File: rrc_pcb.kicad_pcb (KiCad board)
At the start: 2 copper layers, 139 x 50.8 mm, 13 parts, among them J1 Voltage Regulator Input, J2 Conn_01x03_Male, U1 ADXL357Z, U2 Teensy3.6-teensy, U3 BN220-GPS, U4 MS5611, U5 logo

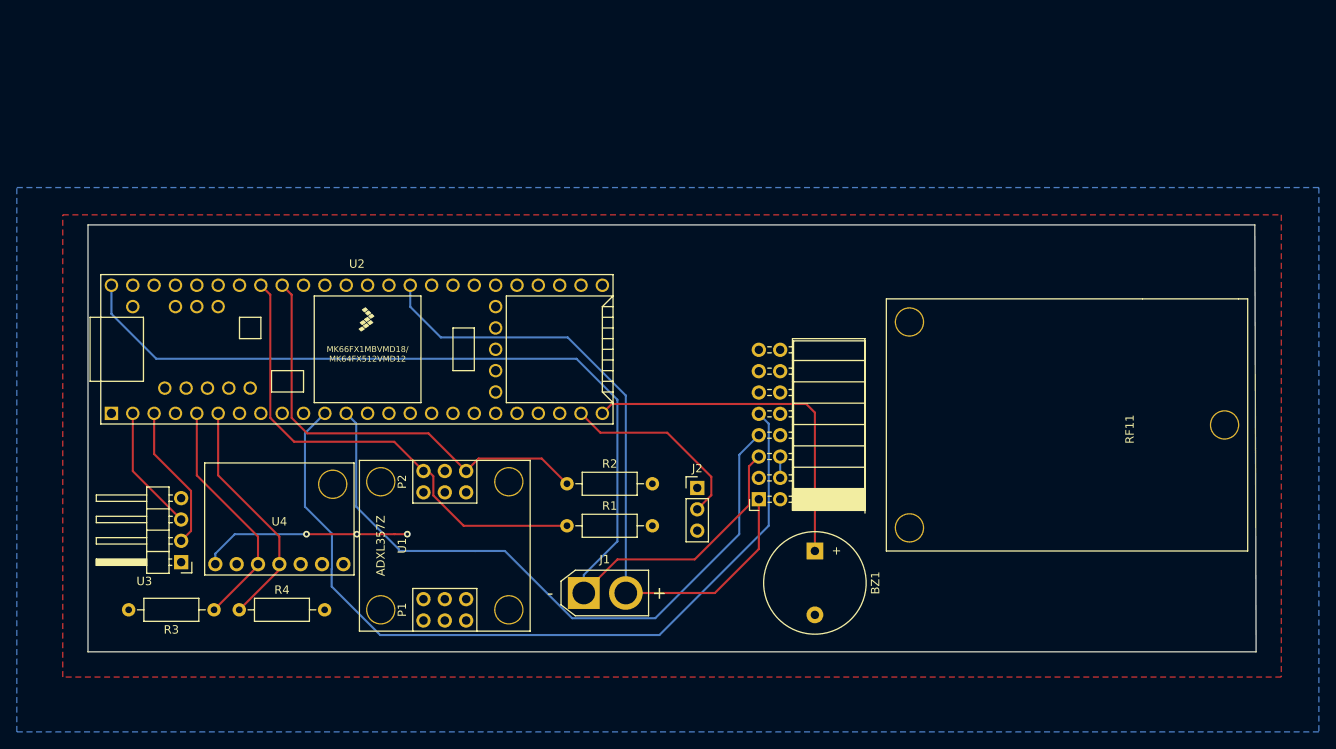
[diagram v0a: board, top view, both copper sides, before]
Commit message: fixed pcb trace issues
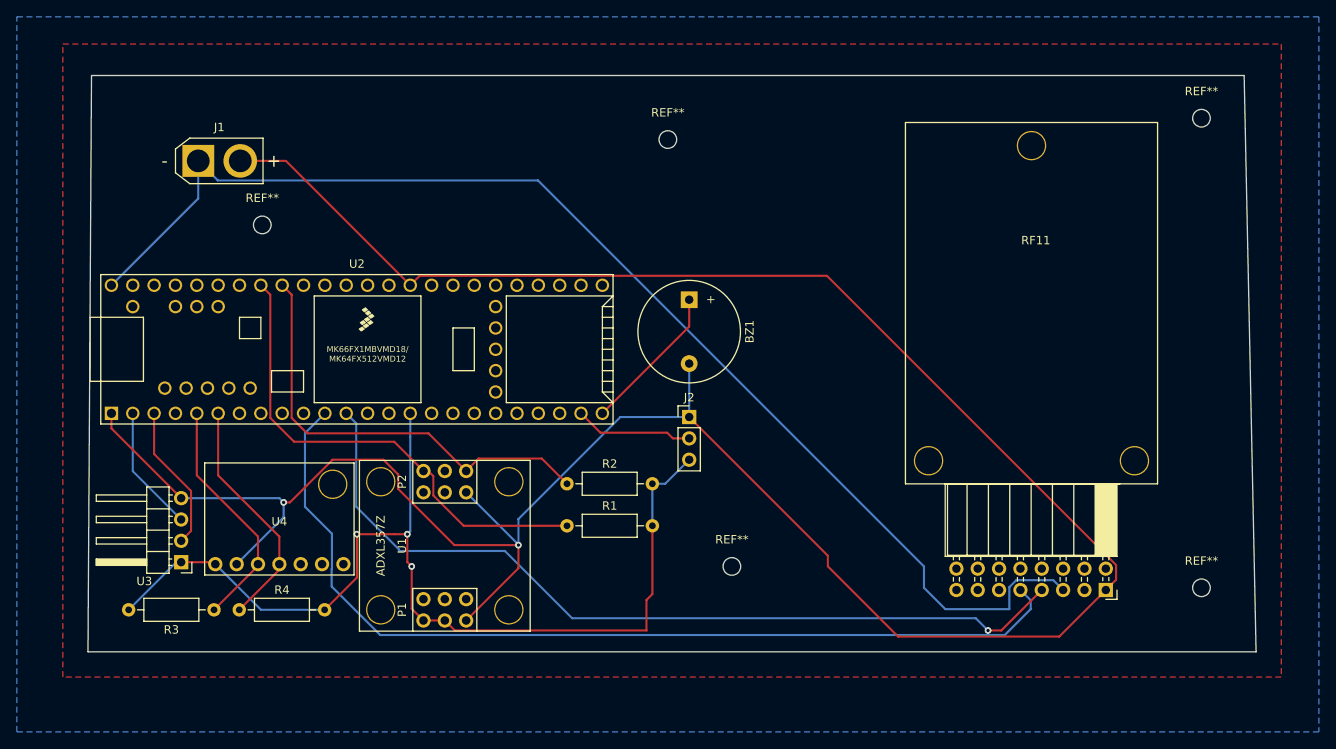
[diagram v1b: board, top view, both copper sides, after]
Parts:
- added REF**: MountingHole_2.1mm, MountingHole:MountingHole_2.1mm, F.Cu at (134.6, 116.8)
- added REF**: MountingHole_2.1mm, MountingHole:MountingHole_2.1mm, F.Cu at (78.7, 76.2)
- added REF**: MountingHole_2.1mm, MountingHole:MountingHole_2.1mm, F.Cu at (190.5, 63.5)
- added REF**: MountingHole_2.1mm, MountingHole:MountingHole_2.1mm, F.Cu at (127.0, 66.0)
- added REF**: MountingHole_2.1mm, MountingHole:MountingHole_2.1mm, F.Cu at (190.5, 119.4)
- moved J1 68.9 mm to (71.1, 68.6)
- moved BZ1 33.4 mm to (129.5, 85.1)
- moved RF11 22.1 mm to (155.3, 107.0), turned to 0 degrees
- moved U5 18.7 mm to (170.2, 83.8)
- moved J2 8.49 mm to (129.5, 99.1)
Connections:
- RF11 pad 10: Net-(RF11-Pad10) -> unconnected-(RF11-Pad10)
- RF11 pad 11: Net-(RF11-Pad11) -> unconnected-(RF11-Pad11)
- RF11 pad 12: Net-(RF11-Pad12) -> unconnected-(RF11-Pad12)
- RF11 pad 13: Net-(RF11-Pad13) -> unconnected-(RF11-Pad13)
- RF11 pad 14: Net-(RF11-Pad14) -> unconnected-(RF11-Pad14)
- RF11 pad 15: Net-(RF11-Pad15) -> unconnected-(RF11-Pad15)
- RF11 pad 16: Net-(RF11-Pad16) -> unconnected-(RF11-Pad16)
- RF11 pad 2: Net-(RF11-Pad2) -> unconnected-(RF11-Pad2)
- RF11 pad 3: Net-(RF11-Pad3) -> unconnected-(RF11-Pad3)
- RF11 pad 8: Net-(RF11-Pad8) -> unconnected-(RF11-Pad8)
- U1 pad 10: Net-(U1-Pad10) -> unconnected-(U1-Pad10)
- U1 pad 2: Net-(U1-Pad2) -> unconnected-(U1-Pad2)
- U1 pad 4: Net-(U1-Pad4) -> unconnected-(U1-Pad4)
- U1 pad 6: Net-(U1-Pad6) -> unconnected-(U1-Pad6)
- U1 pad 7: Net-(U1-Pad7) -> unconnected-(U1-Pad7)
- U1 pad 9: Net-(U1-Pad9) -> unconnected-(U1-Pad9)
- U2 pad 10: Net-(U2-Pad10) -> unconnected-(U2-Pad10)
- U2 pad 13: Net-(U2-Pad13) -> unconnected-(U2-Pad13)
- U2 pad 14: Net-(U2-Pad14) -> unconnected-(U2-Pad14)
- U2 pad 16: Net-(U2-Pad16) -> unconnected-(U2-Pad16)
- U2 pad 17: Net-(U2-Pad17) -> unconnected-(U2-Pad17)
- U2 pad 18: Net-(U2-Pad18) -> unconnected-(U2-Pad18)
- U2 pad 19: Net-(U2-Pad19) -> unconnected-(U2-Pad19)
- U2 pad 20: Net-(U2-Pad20) -> unconnected-(U2-Pad20)
- U2 pad 21: Net-(U2-Pad21) -> unconnected-(U2-Pad21)
- U2 pad 22: Net-(U2-Pad22) -> unconnected-(U2-Pad22)
- U2 pad 25: Net-(U2-Pad25) -> unconnected-(U2-Pad25)
- U2 pad 26: Net-(U2-Pad26) -> unconnected-(U2-Pad26)
- U2 pad 27: Net-(U2-Pad27) -> unconnected-(U2-Pad27)
- U2 pad 28: Net-(U2-Pad28) -> unconnected-(U2-Pad28)
- U2 pad 29: Net-(U2-Pad29) -> unconnected-(U2-Pad29)
- U2 pad 30: Net-(U2-Pad30) -> unconnected-(U2-Pad30)
- U2 pad 31: Net-(U2-Pad31) -> unconnected-(U2-Pad31)
- U2 pad 32: Net-(U2-Pad32) -> unconnected-(U2-Pad32)
- U2 pad 33: Net-(U2-Pad33) -> unconnected-(U2-Pad33)
- U2 pad 34: Net-(U2-Pad34) -> unconnected-(U2-Pad34)
- U2 pad 35: Net-(U2-Pad35) -> unconnected-(U2-Pad35)
- U2 pad 36: Net-(U2-Pad36) -> unconnected-(U2-Pad36)
- U2 pad 37: Net-(U2-Pad37) -> unconnected-(U2-Pad37)
- U2 pad 38: Net-(U2-Pad38) -> unconnected-(U2-Pad38)
- U2 pad 4: Net-(U2-Pad4) -> unconnected-(U2-Pad4)
- U2 pad 40: Net-(U2-Pad40) -> unconnected-(U2-Pad40)
- U2 pad 41: Net-(U2-Pad41) -> unconnected-(U2-Pad41)
- U2 pad 42: Net-(U2-Pad42) -> unconnected-(U2-Pad42)
- U2 pad 43: Net-(U2-Pad43) -> unconnected-(U2-Pad43)
- U2 pad 44: Net-(U2-Pad44) -> unconnected-(U2-Pad44)
- U2 pad 47: Net-(U2-Pad47) -> unconnected-(U2-Pad47)
- U2 pad 48: Net-(U2-Pad48) -> unconnected-(U2-Pad48)
- U2 pad 49: Net-(U2-Pad49) -> unconnected-(U2-Pad49)
- U2 pad 50: Net-(U2-Pad50) -> unconnected-(U2-Pad50)
- U2 pad 51: Net-(U2-Pad51) -> unconnected-(U2-Pad51)
- U2 pad 52: Net-(U2-Pad52) -> unconnected-(U2-Pad52)
- U2 pad 54: Net-(U2-Pad54) -> unconnected-(U2-Pad54)
- U2 pad 55: Net-(U2-Pad55) -> unconnected-(U2-Pad55)
- U2 pad 56: Net-(U2-Pad56) -> unconnected-(U2-Pad56)
- U2 pad 57: Net-(U2-Pad57) -> unconnected-(U2-Pad57)
- U2 pad 7: Net-(U2-Pad7) -> unconnected-(U2-Pad7)
- U2 pad 8: Net-(U2-Pad8) -> unconnected-(U2-Pad8)
- U2 pad 9: Net-(U2-Pad9) -> unconnected-(U2-Pad9)
- U4 pad 5: Net-(U4-Pad5) -> unconnected-(U4-Pad5)
- U4 pad 6: Net-(U4-Pad6) -> unconnected-(U4-Pad6)
- U4 pad 7: Net-(U4-Pad7) -> unconnected-(U4-Pad7)
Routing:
- net T_GND: track 0.00 -> 191.4 mm, vias 0 -> 2
- net T_VCC: track 25.1 -> 120.9 mm
- net GND: track 80.0 -> 128.2 mm
- net VCC: track 122.8 -> 149.0 mm
- net Net-(BZ1-Pad1): track 42.6 -> 17.8 mm
- net Net-(RF11-Pad7): track 79.8 -> 101.5 mm, vias 0 -> 1
- net Net-(RF11-Pad9): track 96.5 -> 112.6 mm
- net Net-(J2-Pad2): track 23.2 -> 14.1 mm
- net Net-(RF11-Pad4): track 2.54 -> 0.00 mm
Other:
- board size 139 x 50.8 mm -> 139 x 68.6 mm
- net class Default removed
